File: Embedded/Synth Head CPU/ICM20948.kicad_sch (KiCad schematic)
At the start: 4 parts, among them U1 ICM-20948

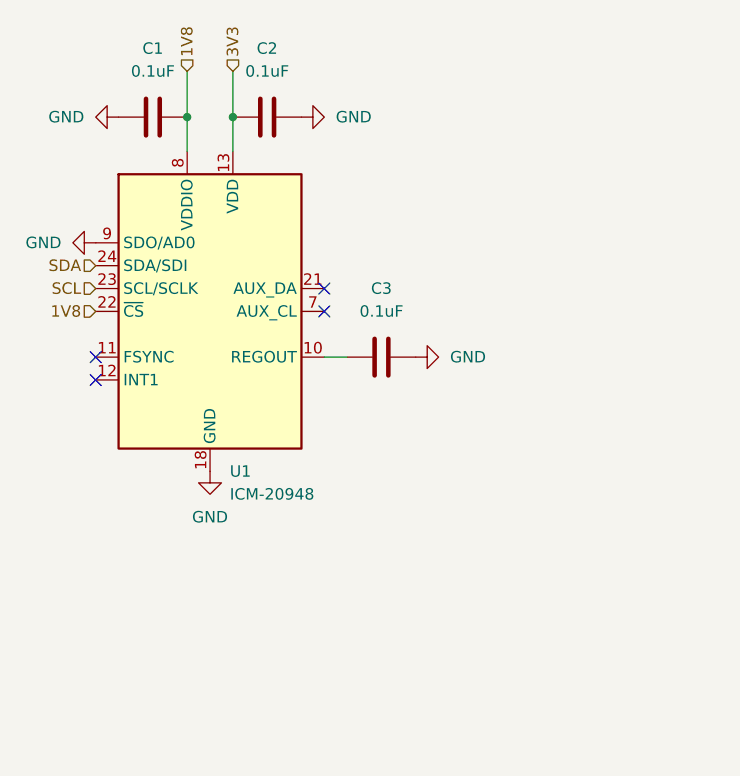
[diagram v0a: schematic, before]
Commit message: Prepared All Main Boards for PCB Creation
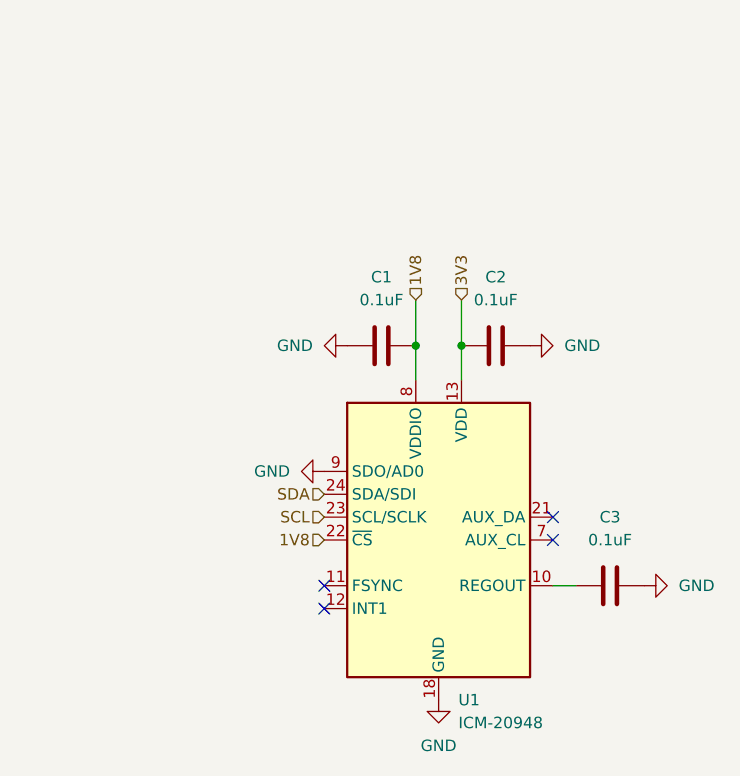
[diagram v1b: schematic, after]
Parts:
- C1, C2, C3: footprint (none) -> Capacitor_SMD:C_0603_1608Metric_Pad1.08x0.95mm_HandSolder
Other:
- moved on the sheet: C1, C2, C3, U1
